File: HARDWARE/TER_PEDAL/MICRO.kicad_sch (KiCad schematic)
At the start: 20 parts, among them J1 DEBUG, SW1 RST, U1 STM32F103C8Tx, Y1 8mHz

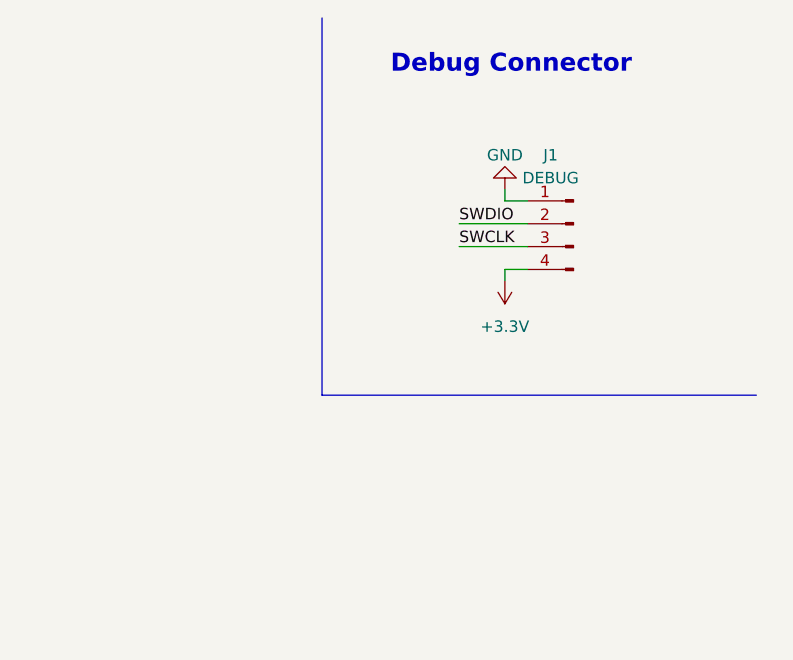
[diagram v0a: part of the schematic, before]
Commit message: Cabiado esquematico, falta layout
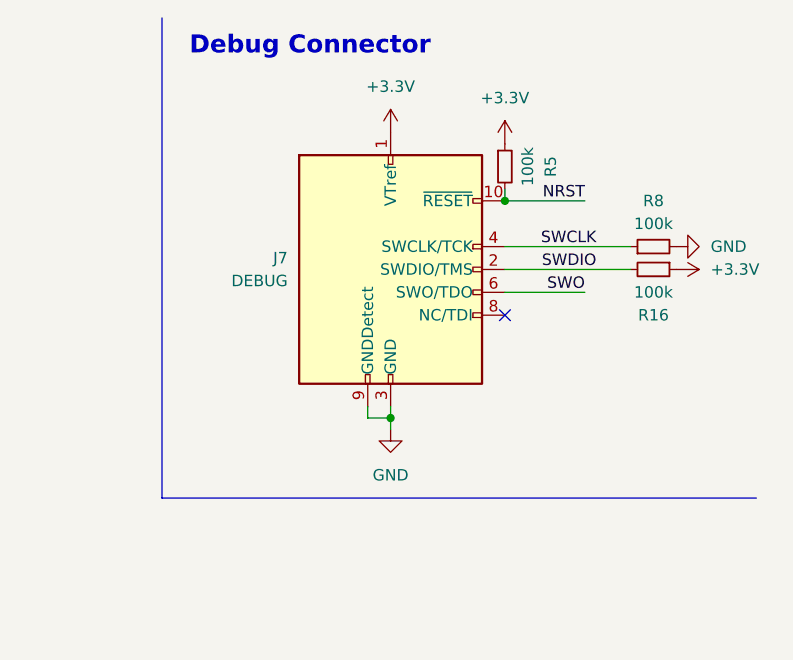
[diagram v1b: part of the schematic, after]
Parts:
- removed J1: DEBUG, Connector_PinHeader_2.00mm:PinHeader_1x04_P2.00mm_Vertical, symbol Connector:Conn_01x04_Male
- added J7: DEBUG, Connector_PinHeader_1.27mm:PinHeader_2x05_P1.27mm_Vertical, symbol Connector:Conn_ARM_JTAG_SWD_10
- added R16, R5, R8: 100k, Resistor_SMD:R_0603_1608Metric, symbol Device:R_Small
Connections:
- net +3.3V: now also J7.1 (VTref), R16.1, R5.1
- net GND: now also J7.3 (GND), J7.5 (GND), J7.9 (GNDDetect), R8.2
- net NRST: now also J7.10 (~{RESET}), R5.2
- net SWCLK: now also J7.4 (SWCLK/TCK), R8.1
- net SWDIO: now also J7.2 (SWDIO/TMS), R16.2
- new net SWO: J7.6 (SWO/TDO)
- no-connect marks 24 -> 25
